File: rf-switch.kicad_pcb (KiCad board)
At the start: 2 copper layers, 1 part

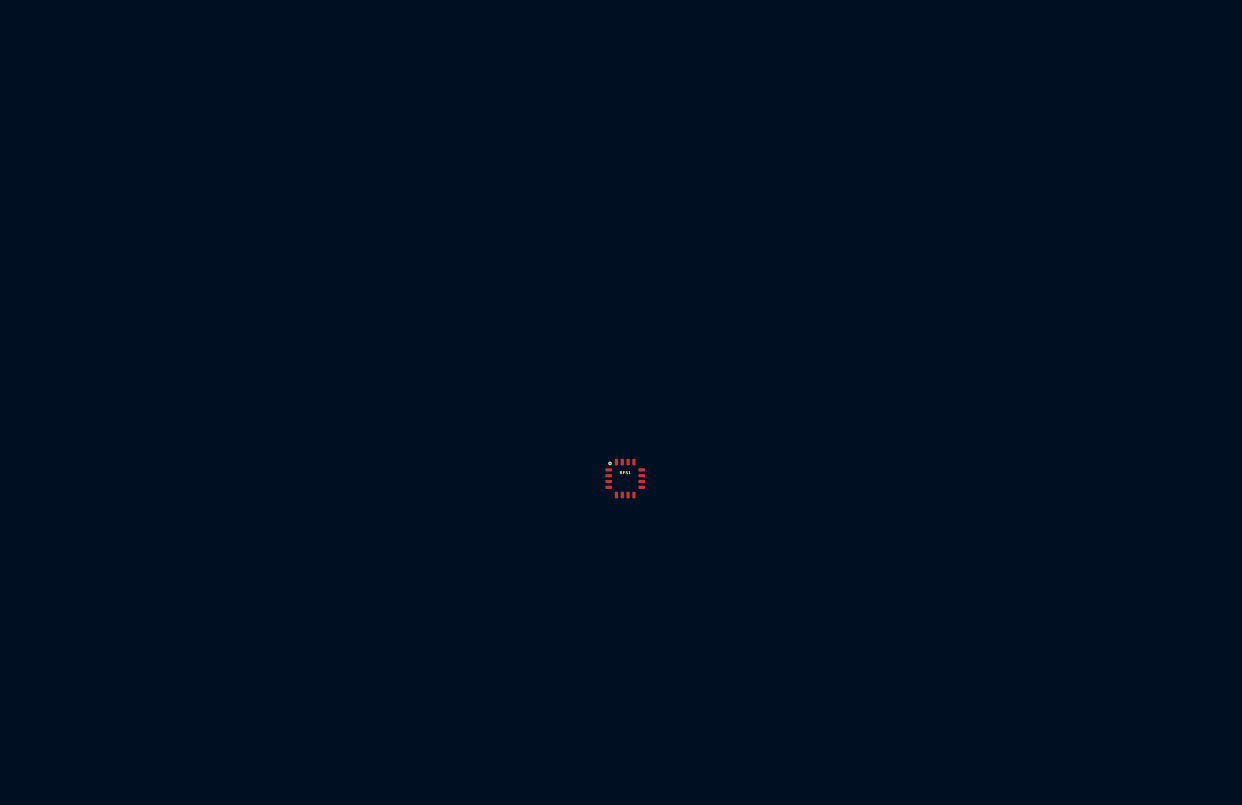
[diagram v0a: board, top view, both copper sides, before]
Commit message: Started PCB Layout
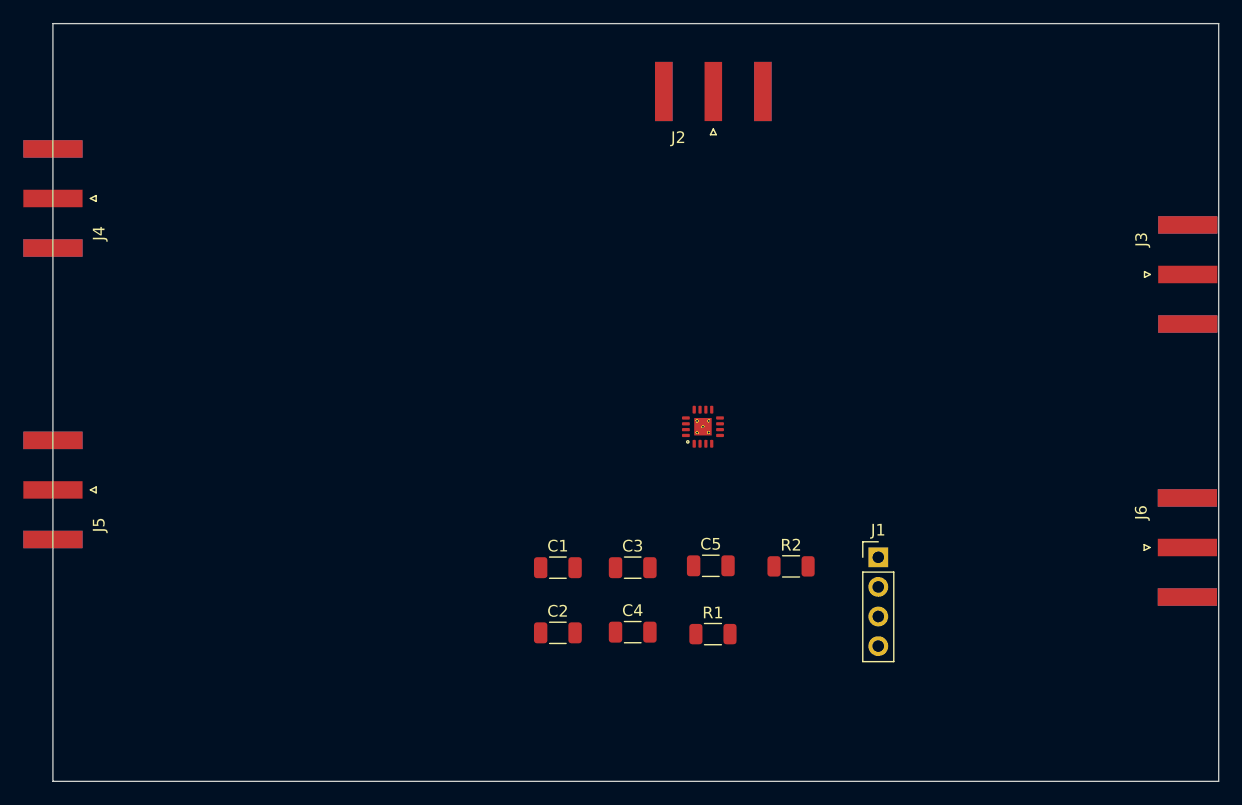
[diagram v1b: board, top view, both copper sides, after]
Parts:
- removed RFS1: ~, PE42440_rf_switch:PE42440
- added C1: 0.01u, Capacitor_SMD:C_1206_3216Metric, F.Cu at (143.3, 106.7)
- added C2: 0.01u, Capacitor_SMD:C_1206_3216Metric, F.Cu at (143.3, 112.3)
- added C3: 10u, Capacitor_SMD:C_1206_3216Metric, F.Cu at (149.7, 106.7)
- added C4: 0.01u, Capacitor_SMD:C_1206_3216Metric, F.Cu at (149.7, 112.2)
- added C5: 0.01u, Capacitor_SMD:C_1206_3216Metric, F.Cu at (156.4, 106.5)
- added IC1: PE42440MLBB-Z, PE42440_rf_switch:PE42440, F.Cu at (155.8, 94.6)
- added J1: Conn_01x04_Pin, Connector_PinHeader_2.54mm:PinHeader_1x04_P2.54mm_Vertical, F.Cu at (170.8, 105.8)
- added J2: Conn_Coaxial_Small, Connector_Coaxial:SMA_Amphenol_132289_EdgeMount, F.Cu at (156.7, 65.8)
- added J3: Conn_Coaxial_Small, Connector_Coaxial:SMA_Amphenol_132289_EdgeMount, F.Cu at (197.3, 81.5)
- added J4: Conn_Coaxial_Small, Connector_Coaxial:SMA_Amphenol_132289_EdgeMount, F.Cu at (100.0, 75.0)
- added J5: Conn_Coaxial_Small, Connector_Coaxial:SMA_Amphenol_132289_EdgeMount, F.Cu at (100.0, 100.0)
- added J6: Conn_Coaxial_Small, Connector_Coaxial:SMA_Amphenol_132289_EdgeMount, F.Cu at (197.3, 104.9)
- added R1: 1M, Resistor_SMD:R_1206_3216Metric, F.Cu at (156.6, 112.4)
- added R2: 1M, Resistor_SMD:R_1206_3216Metric, F.Cu at (163.3, 106.6)
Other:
- board outline added: 100 x 65 mm
